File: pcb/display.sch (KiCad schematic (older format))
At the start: 4 parts

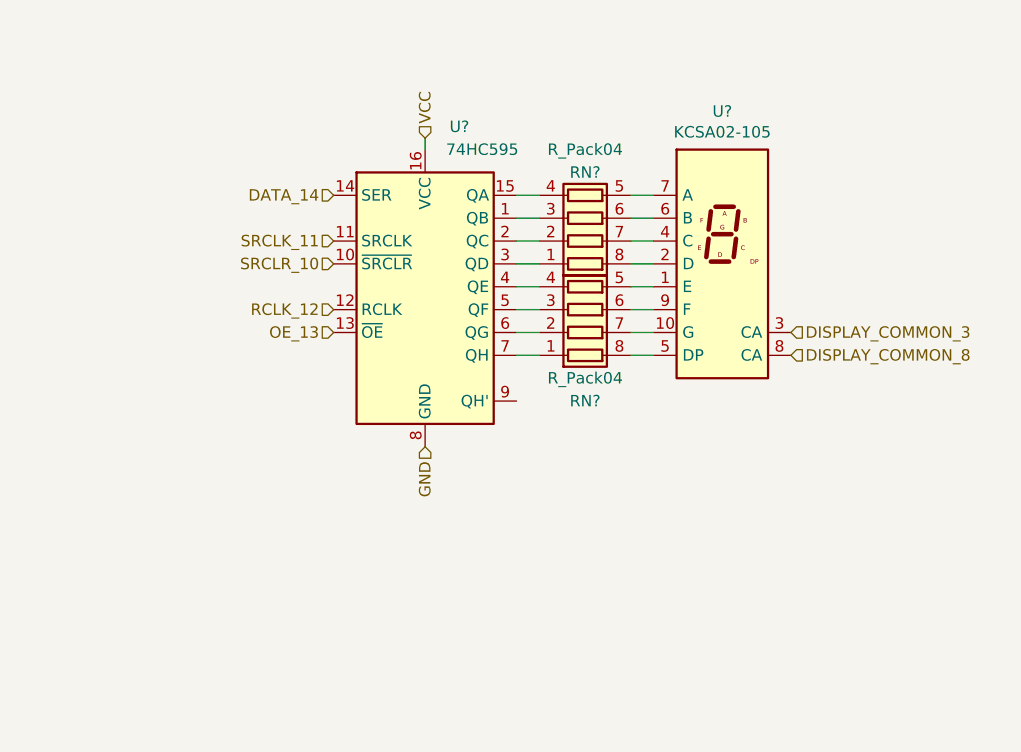
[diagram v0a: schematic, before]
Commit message: Redesign PCB
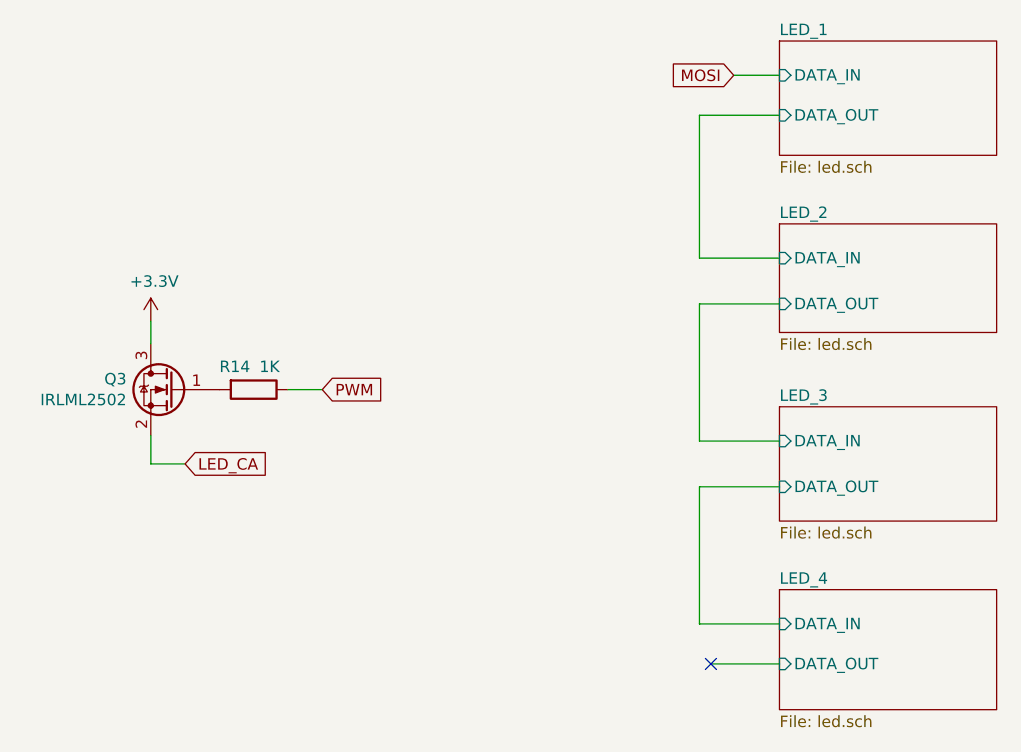
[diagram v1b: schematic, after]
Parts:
- removed RN? (x2): R_Pack04, Resistor_SMD:R_Array_Convex_4x1206, symbol Device:R_Pack04
- removed U?: 74HC595, Package_SO:SOIC-16W_7.5x10.3mm_P1.27mm, symbol 74xx:74HC595
- removed U?: KCSA02-105, Display_7Segment:7SegmentLED_LTS6760_LTS6780, symbol Display_Character:KCSA02-105
- added Q3: IRLML2502, Package_TO_SOT_SMD:SOT-23, symbol Device:Q_NMOS_GSD
- added R14: 1K, Resistor_SMD:R_0805_2012Metric_Pad1.15x1.40mm_HandSolder, symbol Device:R
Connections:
- new net: Q3.1 (G), R14.2
- new net +3V3: Q3.3 (D)
- new net LED_CA: Q3.2 (S)
- new net PWM: R14.1
- no-connect marks 0 -> 1
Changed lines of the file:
@@
 $Descr A4 11693 8268
 encoding utf-8
-Sheet 2 2
+Sheet 5 10
 Title ""
 Date ""
@@
 $EndDescr
 $Comp
-L 74xx:74HC595 U?
-U 1 1 5BFD7445
-P 4950 3400
-AR Path="/5BFD7445" Ref="U?"  Part="1"
-AR Path="/5BFCEFC0/5BFD7445" Ref="U?"  Part="1"
-F 0 "U?" H 5100 4100 50  0000 C CNN
-F 1 "74HC595" H 5200 4000 50  0000 C CNN
-F 2 "Package_SO:SOIC-16W_7.5x10.3mm_P1.27mm" H 4950 3400 50  0001 C CNN
-F 3 "http://www.ti.com/lit/ds/symlink/sn74hc595.pdf" H 4950 3400 50  0001 C CNN
-	1    4950 3400
+L Device:Q_NMOS_GSD Q3
+U 1 1 5C95568F
+P 3850 3850
+F 0 "Q3" H 4056 3896 50  0000 L CNN
+F 1 "IRLML2502" H 4056 3805 50  0000 L CNN
+F 2 "Package_TO_SOT_SMD:SOT-23" H 4050 3950 50  0001 C CNN
+F 3 "https://static.chipdip.ru/lib/144/DOC000144667.pdf" H 3850 3850 50  0001 C CNN
+	1    3850 3850
+	-1   0    0    -1
+$EndComp
+$Comp
+L power:+3.3V #PWR033
+U 1 1 5C955696
+P 3750 3550
+F 0 "#PWR033" H 3750 3400 50  0001 C CNN
+F 1 "+3.3V" H 3765 3723 50  0000 C CNN
+F 2 "" H 3750 3550 50  0001 C CNN
+F 3 "" H 3750 3550 50  0001 C CNN
+	1    3750 3550
 	1    0    0    -1
 $EndComp
 $Comp
-L Device:R_Pack04 RN?
-U 1 1 5BFD744C
-P 5650 3100
-AR Path="/5BFD744C" Ref="RN?"  Part="1"
-AR Path="/5BFCEFC0/5BFD744C" Ref="RN?"  Part="1"
-F 0 "RN?" V 5850 3100 50  0000 C CNN
-F 1 "R_Pack04" V 5950 3100 50  0000 C CNN
-F 2 "Resistor_SMD:R_Array_Convex_4x1206" V 5925 3100 50  0001 C CNN
-F 3 "" H 5650 3100 50  0001 C CNN
-	1    5650 3100
-	0    1    -1   0
+L Device:R R14
+U 1 1 5C95569C
+P 4200 3850
+F 0 "R14" V 4100 3700 50  0000 L CNN
+F 1 "1K" V 4100 3875 50  0000 L CNN
+F 2 "Resistor_SMD:R_0805_2012Metric_Pad1.15x1.40mm_HandSolder" V 4130 3850 50  0001 C CNN
+F 3 "~" H 4200 3850 50  0001 C CNN
+	1    4200 3850
+	0    1    1    0
 $EndComp
-$Comp
-L Device:R_Pack04 RN?
-U 1 1 5BFD7453
-P 5650 3500
-AR Path="/5BFD7453" Ref="RN?"  Part="1"
-AR Path="/5BFCEFC0/5BFD7453" Ref="RN?"  Part="1"
-F 0 "RN?" V 5250 3500 50  0000 C CNN
-F 1 "R_Pack04" V 5350 3500 50  0000 C CNN
-F 2 "Resistor_SMD:R_Array_Convex_4x1206" V 5925 3500 50  0001 C CNN
-F 3 "~" H 5650 3500 50  0001 C CNN
-	1    5650 3500
-	0    1    -1   0
-$EndComp
-$Comp
-L Display_Character:KCSA02-105 U?
-U 1 1 5BFD745A
-P 6250 3300
-AR Path="/5BFD745A" Ref="U?"  Part="1"
-AR Path="/5BFCEFC0/5BFD745A" Ref="U?"  Part="1"
-F 0 "U?" H 6250 3967 50  0000 C CNN
-F 1 "KCSA02-105" H 6250 3876 50  0000 C CNN
-F 2 "Display_7Segment:7SegmentLED_LTS6760_LTS6780" H 6250 2700 50  0001 C CNN
-F 3 "http://www.kingbright.com/attachments/file/psearch/000/00/00/KCSA02-105(Ver.10A).pdf" H 5750 3775 50  0001 L CNN
-	1    6250 3300
-	1    0    0    -1
-$EndComp
+Text GLabel 4500 3850 2    50   Input ~ 0
+PWM
 Wire Wire Line
-	5350 3000 5450 3000
+	4500 3850 4350 3850
+$Sheet
+S 6500 2325 950  500
+U 5C9556A3
+F0 "LED_1" 50
+F1 "led.sch" 50
+F2 "DATA_IN" I L 6500 2475 50
+F3 "DATA_OUT" I L 6500 2650 50
+$EndSheet
+$Sheet
+S 6500 3125 950  475
+U 5C9556A7
+F0 "LED_2" 50
+F1 "led.sch" 50
+F2 "DATA_IN" I L 6500 3275 50
+F3 "DATA_OUT" I L 6500 3475 50
+$EndSheet
+$Sheet
+S 6500 3925 950  500
+U 5C9556AB
+F0 "LED_3" 50
+F1 "led.sch" 50
+F2 "DATA_IN" I L 6500 4075 50
+F3 "DATA_OUT" I L 6500 4275 50
+$EndSheet
 Wire Wire Line
-	5350 3100 5450 3100
+	6500 2650 6150 2650
+Text GLabel 6300 2475 0    50   Input ~ 0
+MOSI
 Wire Wire Line
-	5350 3200 5450 3200
+	6300 2475 6500 2475
 Wire Wire Line
-	5350 3400 5450 3400
+	3750 3550 3750 3650
+Text GLabel 3900 4175 2    50   Input ~ 0
+LED_CA
+$Sheet
+S 6500 4725 950  525
+U 5C9556BE
+F0 "LED_4" 50
+F1 "led.sch" 50
+F2 "DATA_IN" I L 6500 4875 50
+F3 "DATA_OUT" I L 6500 5050 50
+$EndSheet
 Wire Wire Line
-	5350 3500 5450 3500
+	3750 4050 3750 4175
 Wire Wire Line
-	5350 3600 5450 3600
+	3750 4175 3900 4175
 Wire Wire Line
-	5350 3700 5450 3700
+	6150 2650 6150 3275
 Wire Wire Line
-	4950 2750 4950 2800
+	6150 3275 6500 3275
 Wire Wire Line
-	5850 3000 5950 3000
+	6500 3475 6150 3475
 Wire Wire Line
-	5850 3100 5950 3100
+	6150 3475 6150 4075
 Wire Wire Line
-	5850 3700 5950 3700
+	6150 4075 6500 4075
 Wire Wire Line
-	5850 3600 5950 3600
+	6500 4275 6150 4275
 Wire Wire Line
-	5850 3500 5950 3500
+	6150 4275 6150 4875
 Wire Wire Line
-	5850 3400 5950 3400
+	6150 4875 6500 4875
+NoConn ~ 6200 5050
 Wire Wire Line
-	5850 3200 5950 3200
-Wire Wire Line
-	5350 3300 5450 3300
-Wire Wire Line
-	5850 3300 5950 3300
-Text HLabel 4950 4100 3    50   Input ~ 0
-GND
-Text HLabel 6550 3700 2    50   Input ~ 0
-DISPLAY_COMMON_8
-Text HLabel 4950 2750 1    50   Input ~ 0
-VCC
-Text HLabel 4550 3000 0    50   Input ~ 0
-DATA_14
-Text HLabel 4550 3200 0    50   Input ~ 0
-SRCLK_11
-Text HLabel 4550 3300 0    50   Input ~ 0
-SRCLR_10
-Text HLabel 4550 3500 0    50   Input ~ 0
-RCLK_12
-Text HLabel 4550 3600 0    50   Input ~ 0
-OE_13
-Text HLabel 6550 3600 2    50   Input ~ 0
-DISPLAY_COMMON_3
+	6500 5050 6200 5050
 $EndSCHEMATC
